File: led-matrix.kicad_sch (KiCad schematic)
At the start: 168 parts

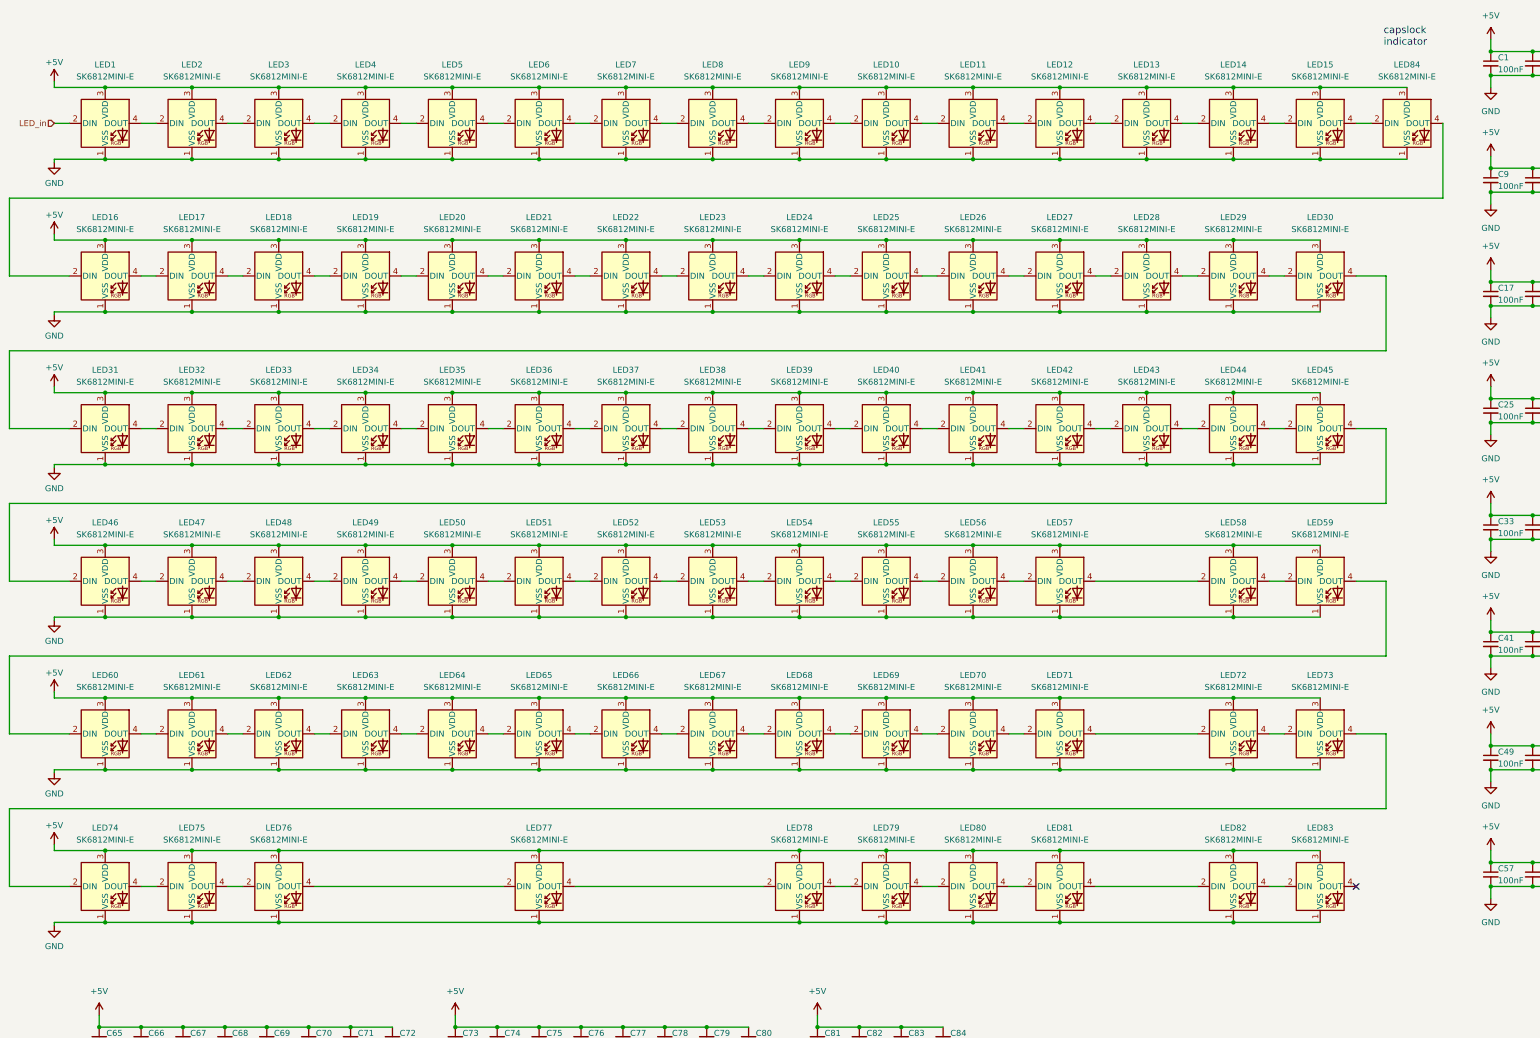
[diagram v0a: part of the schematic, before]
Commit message: completed pcb design
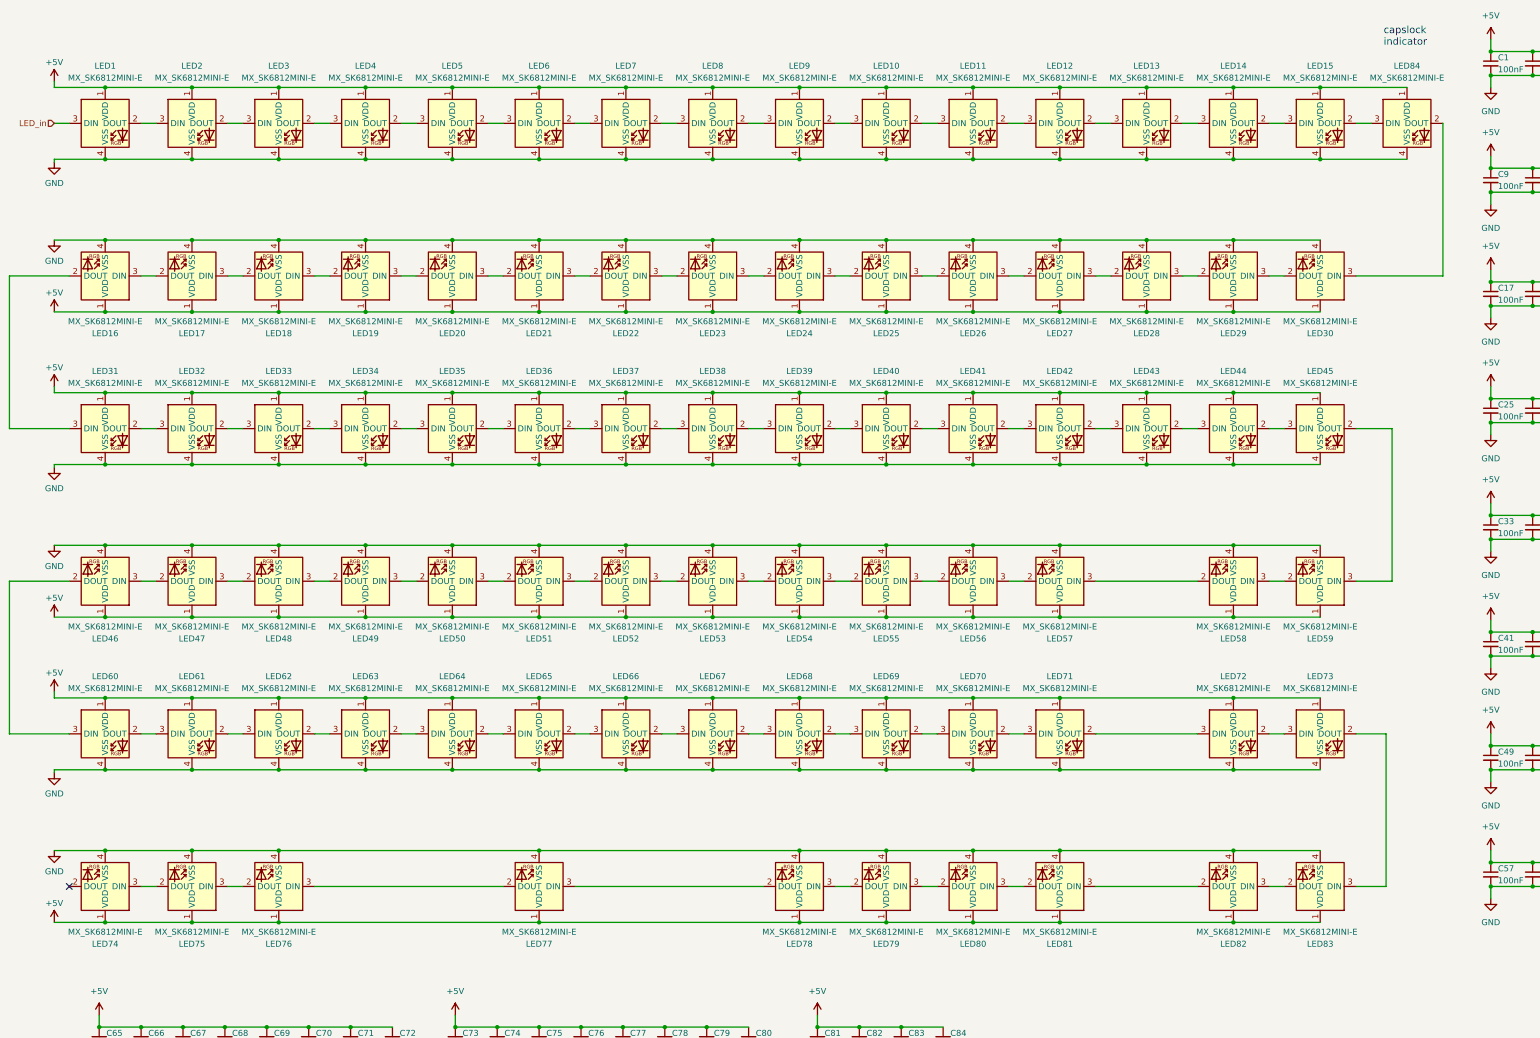
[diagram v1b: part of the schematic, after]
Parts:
- removed LED1, LED10, LED11, LED12, LED13, LED14, LED15, LED16, LED17, LED18, LED19, LED2, LED20, LED21, LED22, LED23, LED24, LED25, LED26, LED27, LED28, LED29, LED3, LED30, LED31, LED32, LED33, LED34, LED35, LED36, LED37, LED38, LED39, LED4, LED40, LED41, LED42, LED43, LED44, LED45, LED46, LED47, LED48, LED49, LED5, LED50, LED51, LED52, LED53, LED54, LED55, LED56, LED57, LED58, LED59, LED6, LED60, LED61, LED62, LED63, LED64, LED65, LED66, LED67, LED68, LED69, LED7, LED70, LED71, LED72, LED73, LED74, LED75, LED76, LED77, LED78, LED79, LED8, LED80, LED81, LED82, LED83, LED84, LED9: SK6812MINI-E, LED_SMD:LED_SK6812MINI-E_3.2x2.8mm_P1.5mm_ReverseMount, symbol LED:SK6812MINI-E
- added LED1, LED10, LED11, LED12, LED13, LED14, LED15, LED2, LED3, LED31, LED32, LED33, LED34, LED35, LED36, LED37, LED38, LED39, LED4, LED40, LED41, LED42, LED43, LED44, LED45, LED5, LED6, LED60, LED61, LED62, LED63, LED64, LED65, LED66, LED67, LED68, LED69, LED7, LED70, LED71, LED72, LED73, LED8, LED84, LED9: MX_SK6812MINI-E, PCM_marbastlib-mx:LED_MX_6028R-ROT, symbol PCM_marbastlib-mx:MX_SK6812MINI-E
- added LED16, LED17, LED18, LED19, LED20, LED21, LED22, LED23, LED24, LED25, LED26, LED27, LED28, LED29, LED30, LED46, LED47, LED48, LED49, LED50, LED51, LED52, LED53, LED54, LED55, LED56, LED57, LED58, LED59, LED74, LED75, LED76, LED77, LED78, LED79, LED80, LED81, LED82, LED83: MX_SK6812MINI-E, PCM_marbastlib-mx:LED_MX_6028R, symbol PCM_marbastlib-mx:MX_SK6812MINI-E
- C1, C10, C11, C12, C13, C14, C15, C16, C17, C18, C19, C2, C20, C21, C22, C23, C24, C25, C26, C27, C28, C29, C3, C30, C31, C32, C33, C34, C35, C36, C37, C38, C39, C4, C40, C41, C42, C43, C44, C45, C46, C47, C48, C49, C5, C50, C51, C52, C53, C54, C55, C56, C57, C58, C59, C6, C60, C61, C62, C63, C64, C65, C66, C67, C68, C69, C7, C70, C71, C72, C73, C74, C75, C76, C77, C78, C79, C8, C80, C81, C82, C83, C84, C9: footprint Capacitor_SMD:C_0402_1005Metric -> smd_silkscreen:C_0402_1005Metric
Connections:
- net +5V: now also LED1.1 (VDD), LED10.1 (VDD), LED11.1 (VDD), LED12.1 (VDD), LED13.1 (VDD), LED14.1 (VDD), LED15.1 (VDD), LED16.1 (VDD), LED17.1 (VDD), LED18.1 (VDD), LED19.1 (VDD), LED2.1 (VDD), LED20.1 (VDD), LED21.1 (VDD), LED22.1 (VDD), LED23.1 (VDD), LED24.1 (VDD), LED25.1 (VDD), LED26.1 (VDD), LED27.1 (VDD), LED28.1 (VDD), LED29.1 (VDD), LED3.1 (VDD), LED30.1 (VDD), LED31.1 (VDD), LED32.1 (VDD), LED33.1 (VDD), LED34.1 (VDD), LED35.1 (VDD), LED36.1 (VDD), LED37.1 (VDD), LED38.1 (VDD), LED39.1 (VDD), LED4.1 (VDD), LED40.1 (VDD), LED41.1 (VDD), LED42.1 (VDD), LED43.1 (VDD), LED44.1 (VDD), LED45.1 (VDD), LED46.1 (VDD), LED47.1 (VDD), LED48.1 (VDD), LED49.1 (VDD), LED5.1 (VDD), LED50.1 (VDD), LED51.1 (VDD), LED52.1 (VDD), LED53.1 (VDD), LED54.1 (VDD), LED55.1 (VDD), LED56.1 (VDD), LED57.1 (VDD), LED58.1 (VDD), LED59.1 (VDD), LED6.1 (VDD), LED60.1 (VDD), LED61.1 (VDD), LED62.1 (VDD), LED63.1 (VDD), LED64.1 (VDD), LED65.1 (VDD), LED66.1 (VDD), LED67.1 (VDD), LED68.1 (VDD), LED69.1 (VDD), LED7.1 (VDD), LED70.1 (VDD), LED71.1 (VDD), LED72.1 (VDD), LED73.1 (VDD), LED74.1 (VDD), LED75.1 (VDD), LED76.1 (VDD), LED77.1 (VDD), LED78.1 (VDD), LED79.1 (VDD), LED8.1 (VDD), LED80.1 (VDD), LED81.1 (VDD), LED82.1 (VDD), LED83.1 (VDD), LED84.1 (VDD), LED9.1 (VDD)
- net GND: now also LED1.4 (VSS), LED10.4 (VSS), LED11.4 (VSS), LED12.4 (VSS), LED13.4 (VSS), LED14.4 (VSS), LED15.4 (VSS), LED16.4 (VSS), LED17.4 (VSS), LED18.4 (VSS), LED19.4 (VSS), LED2.4 (VSS), LED20.4 (VSS), LED21.4 (VSS), LED22.4 (VSS), LED23.4 (VSS), LED24.4 (VSS), LED25.4 (VSS), LED26.4 (VSS), LED27.4 (VSS), LED28.4 (VSS), LED29.4 (VSS), LED3.4 (VSS), LED30.4 (VSS), LED31.4 (VSS), LED32.4 (VSS), LED33.4 (VSS), LED34.4 (VSS), LED35.4 (VSS), LED36.4 (VSS), LED37.4 (VSS), LED38.4 (VSS), LED39.4 (VSS), LED4.4 (VSS), LED40.4 (VSS), LED41.4 (VSS), LED42.4 (VSS), LED43.4 (VSS), LED44.4 (VSS), LED45.4 (VSS), LED46.4 (VSS), LED47.4 (VSS), LED48.4 (VSS), LED49.4 (VSS), LED5.4 (VSS), LED50.4 (VSS), LED51.4 (VSS), LED52.4 (VSS), LED53.4 (VSS), LED54.4 (VSS), LED55.4 (VSS), LED56.4 (VSS), LED57.4 (VSS), LED58.4 (VSS), LED59.4 (VSS), LED6.4 (VSS), LED60.4 (VSS), LED61.4 (VSS), LED62.4 (VSS), LED63.4 (VSS), LED64.4 (VSS), LED65.4 (VSS), LED66.4 (VSS), LED67.4 (VSS), LED68.4 (VSS), LED69.4 (VSS), LED7.4 (VSS), LED70.4 (VSS), LED71.4 (VSS), LED72.4 (VSS), LED73.4 (VSS), LED74.4 (VSS), LED75.4 (VSS), LED76.4 (VSS), LED77.4 (VSS), LED78.4 (VSS), LED79.4 (VSS), LED8.4 (VSS), LED80.4 (VSS), LED81.4 (VSS), LED82.4 (VSS), LED83.4 (VSS), LED84.4 (VSS), LED9.4 (VSS)
- net LED_in: now also LED1.3 (DIN)
- new net: LED62.2 (DOUT), LED63.3 (DIN)
- new net: LED61.2 (DOUT), LED62.3 (DIN)
- new net: LED15.2 (DOUT), LED84.3 (DIN)
- new net: LED14.2 (DOUT), LED15.3 (DIN)
- new net: LED22.3 (DIN), LED23.2 (DOUT)
- new net: LED23.3 (DIN), LED24.2 (DOUT)
- new net: LED47.3 (DIN), LED48.2 (DOUT)
- new net: LED48.3 (DIN), LED49.2 (DOUT)
- new net: LED16.2 (DOUT), LED31.3 (DIN)
- new net: LED16.3 (DIN), LED17.2 (DOUT)
- new net: LED7.2 (DOUT), LED8.3 (DIN)
- new net: LED6.2 (DOUT), LED7.3 (DIN)
- new net: LED54.3 (DIN), LED55.2 (DOUT)
- new net: LED55.3 (DIN), LED56.2 (DOUT)
- new net: LED80.3 (DIN), LED81.2 (DOUT)
- new net: LED81.3 (DIN), LED82.2 (DOUT)
- new net: LED73.2 (DOUT), LED83.3 (DIN)
- new net: LED72.2 (DOUT), LED73.3 (DIN)
- new net: LED12.2 (DOUT), LED13.3 (DIN)
- new net: LED11.2 (DOUT), LED12.3 (DIN)
- new net: LED56.3 (DIN), LED57.2 (DOUT)
- new net: LED57.3 (DIN), LED58.2 (DOUT)
- new net: LED82.3 (DIN), LED83.2 (DOUT)
- new net: LED21.3 (DIN), LED22.2 (DOUT)
- new net: LED26.3 (DIN), LED27.2 (DOUT)
- new net: LED27.3 (DIN), LED28.2 (DOUT)
- new net: LED28.3 (DIN), LED29.2 (DOUT)
- new net: LED5.2 (DOUT), LED6.3 (DIN)
- new net: LED4.2 (DOUT), LED5.3 (DIN)
- new net: LED17.3 (DIN), LED18.2 (DOUT)
- new net: LED77.3 (DIN), LED78.2 (DOUT)
- new net: LED78.3 (DIN), LED79.2 (DOUT)
- new net: LED71.2 (DOUT), LED72.3 (DIN)
- new net: LED40.2 (DOUT), LED41.3 (DIN)
- new net: LED39.2 (DOUT), LED40.3 (DIN)
- new net: LED8.2 (DOUT), LED9.3 (DIN)
- new net: LED60.2 (DOUT), LED61.3 (DIN)
- new net: LED25.3 (DIN), LED26.2 (DOUT)
- new net: LED10.2 (DOUT), LED11.3 (DIN)
- new net: LED10.3 (DIN), LED9.2 (DOUT)
- new net: LED75.3 (DIN), LED76.2 (DOUT)
- new net: LED76.3 (DIN), LED77.2 (DOUT)
- new net: LED46.2 (DOUT), LED60.3 (DIN)
- new net: LED46.3 (DIN), LED47.2 (DOUT)
- new net: LED13.2 (DOUT), LED14.3 (DIN)
- new net: LED29.3 (DIN), LED30.2 (DOUT)
- new net: LED69.2 (DOUT), LED70.3 (DIN)
- new net: LED68.2 (DOUT), LED69.3 (DIN)
- new net: LED44.2 (DOUT), LED45.3 (DIN)
- new net: LED43.2 (DOUT), LED44.3 (DIN)
- new net: LED49.3 (DIN), LED50.2 (DOUT)
- new net: LED36.2 (DOUT), LED37.3 (DIN)
- new net: LED35.2 (DOUT), LED36.3 (DIN)
- new net: LED74.3 (DIN), LED75.2 (DOUT)
- new net: LED65.2 (DOUT), LED66.3 (DIN)
- new net: LED64.2 (DOUT), LED65.3 (DIN)
- new net: LED66.2 (DOUT), LED67.3 (DIN)
- new net: LED37.2 (DOUT), LED38.3 (DIN)
- new net: LED30.3 (DIN), LED84.2 (DOUT)
- new net: LED79.3 (DIN), LED80.2 (DOUT)
- new net: LED33.2 (DOUT), LED34.3 (DIN)
- new net: LED32.2 (DOUT), LED33.3 (DIN)
- new net: LED58.3 (DIN), LED59.2 (DOUT)
- new net: LED45.2 (DOUT), LED59.3 (DIN)
- new net: LED31.2 (DOUT), LED32.3 (DIN)
- new net: LED38.2 (DOUT), LED39.3 (DIN)
- new net: LED42.2 (DOUT), LED43.3 (DIN)
- new net: LED34.2 (DOUT), LED35.3 (DIN)
- new net: LED20.3 (DIN), LED21.2 (DOUT)
- new net: LED18.3 (DIN), LED19.2 (DOUT)
- new net: LED2.2 (DOUT), LED3.3 (DIN)
- new net: LED1.2 (DOUT), LED2.3 (DIN)
- new net: LED3.2 (DOUT), LED4.3 (DIN)
- new net: LED24.3 (DIN), LED25.2 (DOUT)
- new net: LED63.2 (DOUT), LED64.3 (DIN)
- new net: LED67.2 (DOUT), LED68.3 (DIN)
- new net: LED70.2 (DOUT), LED71.3 (DIN)
- new net: LED50.3 (DIN), LED51.2 (DOUT)
- new net: LED41.2 (DOUT), LED42.3 (DIN)
- new net: LED19.3 (DIN), LED20.2 (DOUT)
- new net: LED53.3 (DIN), LED54.2 (DOUT)
- new net: LED51.3 (DIN), LED52.2 (DOUT)
- new net: LED52.3 (DIN), LED53.2 (DOUT)
